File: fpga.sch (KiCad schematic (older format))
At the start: 58 parts, among them P1 JTAG_CONN, SW2 SW_PUSH, U10 S25FL216K, U12 TLV70012, U13 TLV70025, U14 TLV70012, U2 EP4CE15E22

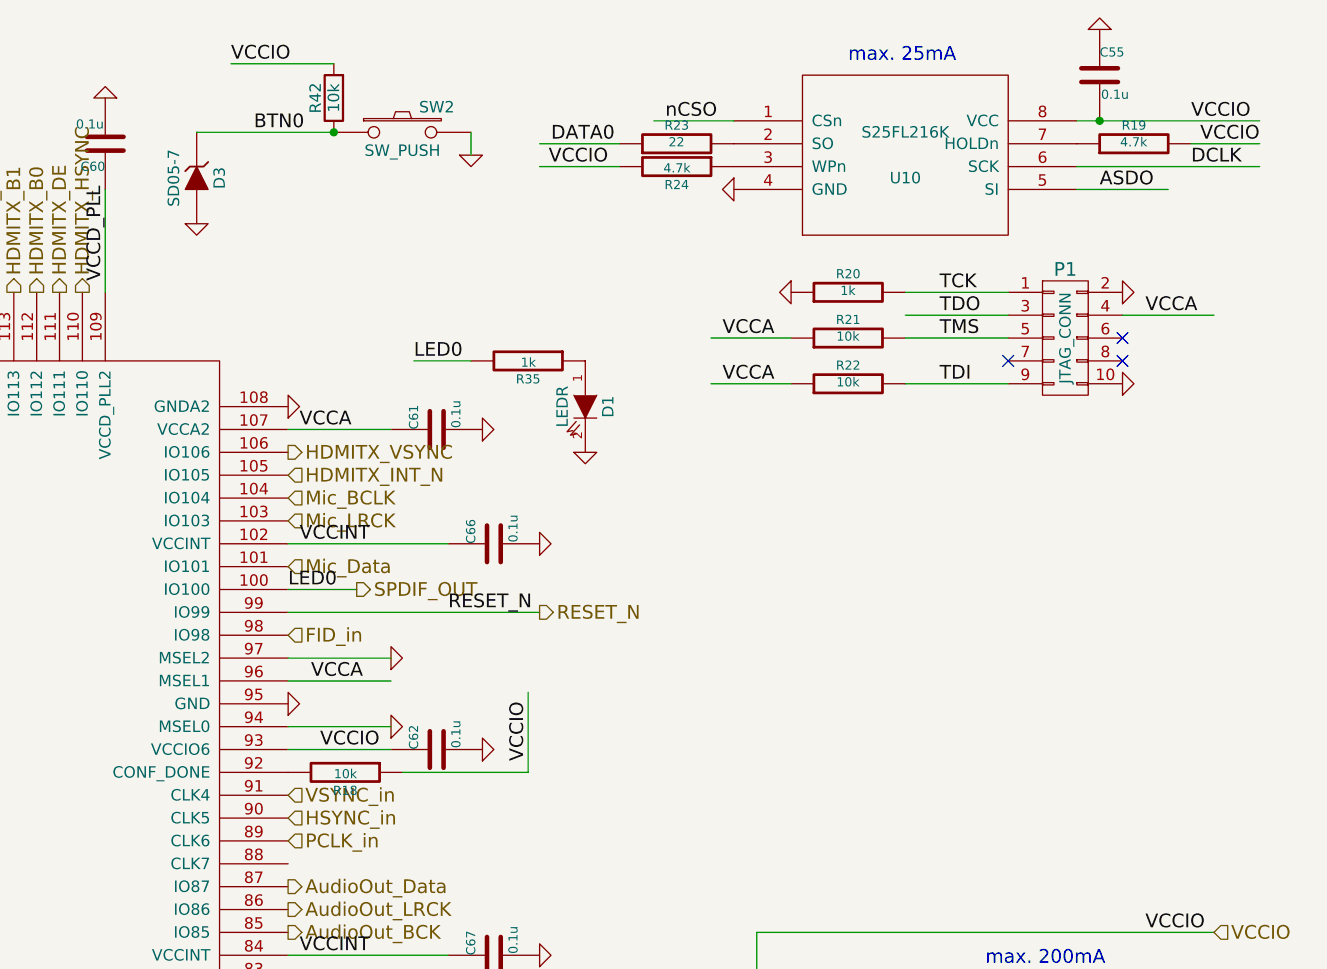
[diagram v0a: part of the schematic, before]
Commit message: update PCB 2
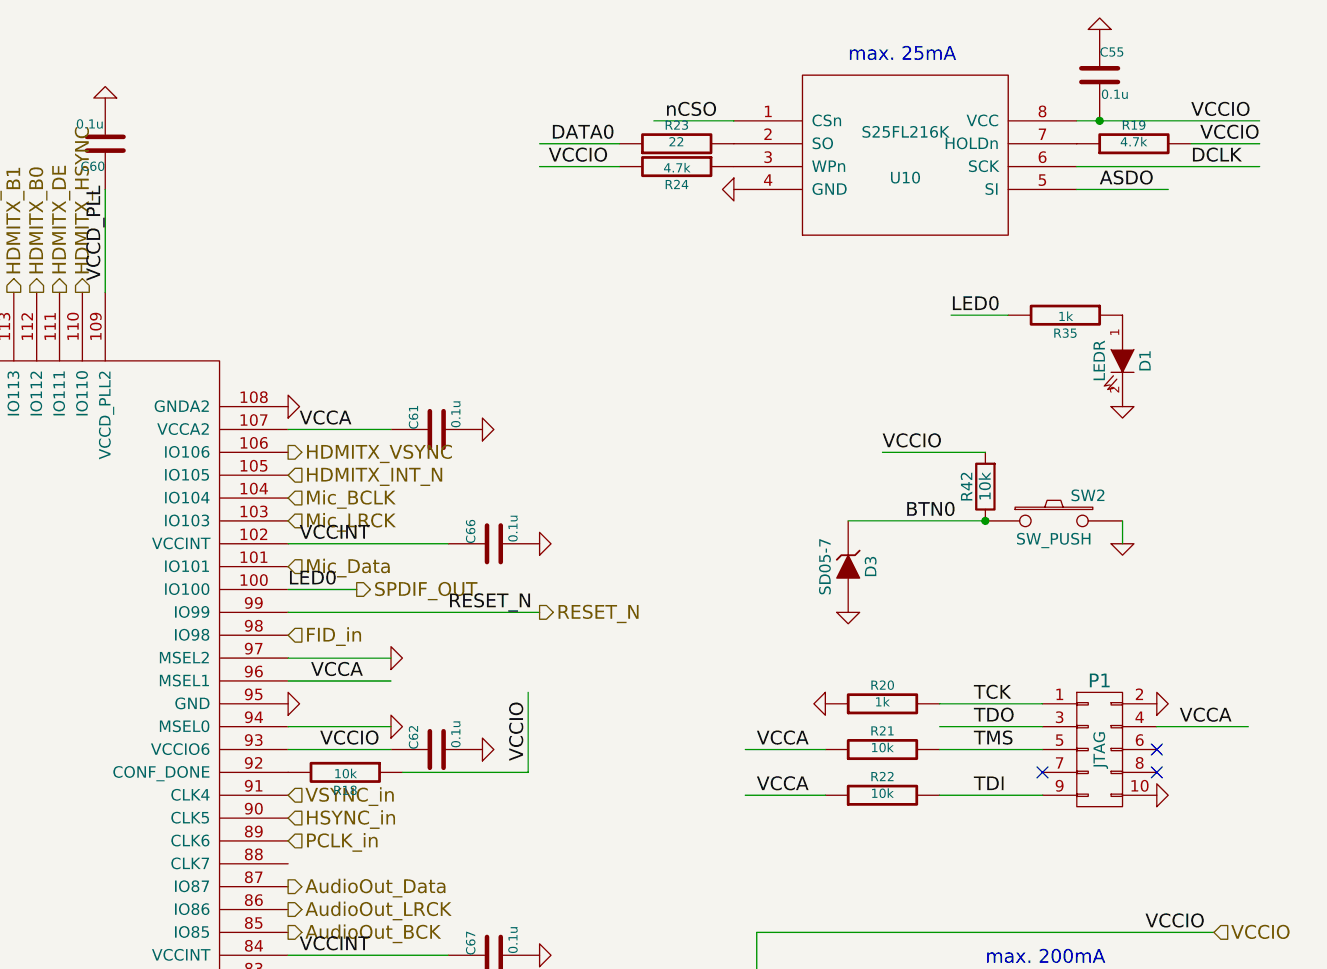
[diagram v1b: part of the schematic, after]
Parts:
- P1: value JTAG_CONN -> JTAG
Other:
- moved on the sheet: D1, D3, P1, R20, R21, R22, R35, R42, SW2
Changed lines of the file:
@@
 L ossc_board-rescue:CONN_02X05 P1
 U 1 1 54FE1877
-P 10200 2050
-F 0 "P1" H 10200 2350 60  0000 C CNN
-F 1 "JTAG_CONN" V 10200 2050 50  0000 C CNN
-F 2 "Connect:VASCH5x2" H 10200 2050 60  0001 C CNN
-F 3 "" H 10200 2050 60  0000 C CNN
-	1    10200 2050
-	1    0    0    -1
-$EndComp
-Text Label 9650 1850 0    60   ~ 0
+P 10350 3850
+F 0 "P1" H 10350 4150 60  0000 C CNN
+F 1 "JTAG" V 10350 3850 50  0000 C CNN
+F 2 "Connect:VASCH5x2" H 10350 3850 60  0001 C CNN
+F 3 "" H 10350 3850 60  0000 C CNN
+	1    10350 3850
+	1    0    0    -1
+$EndComp
+Text Label 9800 3650 0    60   ~ 0
 TCK
-Text Label 9650 1950 0    60   ~ 0
+Text Label 9800 3750 0    60   ~ 0
 TDO
-Text Label 9650 2050 0    60   ~ 0
+Text Label 9800 3850 0    60   ~ 0
 TMS
-Text Label 9650 2250 0    60   ~ 0
+Text Label 9800 4050 0    60   ~ 0
 TDI
 $Comp
 L ossc_board-rescue:GND-RESCUE-ossc_board #PWR048
 U 1 1 54FE19F5
-P 10450 1850
-F 0 "#PWR048" H 10450 1850 30  0001 C CNN
-F 1 "GND" H 10450 1780 30  0001 C CNN
-F 2 "" H 10450 1850 60  0001 C CNN
-F 3 "" H 10450 1850 60  0000 C CNN
-	1    10450 1850
+P 10600 3650
+F 0 "#PWR048" H 10600 3650 30  0001 C CNN
+F 1 "GND" H 10600 3580 30  0001 C CNN
+F 2 "" H 10600 3650 60  0001 C CNN
+F 3 "" H 10600 3650 60  0000 C CNN
+	1    10600 3650
 	0    -1   -1   0
 $EndComp
@@
 L ossc_board-rescue:GND-RESCUE-ossc_board #PWR049
 U 1 1 54FE19FB
-P 10450 2250
-F 0 "#PWR049" H 10450 2250 30  0001 C CNN
-F 1 "GND" H 10450 2180 30  0001 C CNN
-F 2 "" H 10450 2250 60  0001 C CNN
-F 3 "" H 10450 2250 60  0000 C CNN
-	1    10450 2250
+P 10600 4050
+F 0 "#PWR049" H 10600 4050 30  0001 C CNN
+F 1 "GND" H 10600 3980 30  0001 C CNN
+F 2 "" H 10600 4050 60  0001 C CNN
+F 3 "" H 10600 4050 60  0000 C CNN
+	1    10600 4050
 	0    -1   -1   0
 $EndComp
-Text Label 10550 1950 0    60   ~ 0
+Text Label 10700 3750 0    60   ~ 0
 VCCA
 $Comp
 L ossc_board-rescue:R-RESCUE-ossc_board R20
 U 1 1 54FE1A84
-P 9250 1850
-F 0 "R20" V 9330 1850 40  0000 C CNN
-F 1 "1k" V 9257 1851 40  0000 C CNN
-F 2 "Resistor_SMD:R_0603_1608Metric_Pad1.05x0.95mm_HandSolder" V 9180 1850 30  0001 C CNN
-F 3 "~" H 9250 1850 30  0000 C CNN
-	1    9250 1850
+P 9400 3650
+F 0 "R20" V 9480 3650 40  0000 C CNN
+F 1 "1k" V 9407 3651 40  0000 C CNN
+F 2 "Resistor_SMD:R_0603_1608Metric_Pad1.05x0.95mm_HandSolder" V 9330 3650 30  0001 C CNN
+F 3 "~" H 9400 3650 30  0000 C CNN
+	1    9400 3650
 	0    -1   -1   0
 $EndComp
@@
 L ossc_board-rescue:GND-RESCUE-ossc_board #PWR050
 U 1 1 54FE1A96
-P 9000 1850
-F 0 "#PWR050" H 9000 1850 30  0001 C CNN
-F 1 "GND" H 9000 1780 30  0001 C CNN
-F 2 "" H 9000 1850 60  0001 C CNN
-F 3 "" H 9000 1850 60  0000 C CNN
-	1    9000 1850
+P 9150 3650
+F 0 "#PWR050" H 9150 3650 30  0001 C CNN
+F 1 "GND" H 9150 3580 30  0001 C CNN
+F 2 "" H 9150 3650 60  0001 C CNN
+F 3 "" H 9150 3650 60  0000 C CNN
+	1    9150 3650
 	0    1    1    0
 $EndComp
@@
 L ossc_board-rescue:R-RESCUE-ossc_board R21
 U 1 1 54FE1A9C
-P 9250 2050
-F 0 "R21" V 9330 2050 40  0000 C CNN
-F 1 "10k" V 9257 2051 40  0000 C CNN
-F 2 "Resistor_SMD:R_0603_1608Metric_Pad1.05x0.95mm_HandSolder" V 9180 2050 30  0001 C CNN
-F 3 "~" H 9250 2050 30  0000 C CNN
-	1    9250 2050
+P 9400 3850
+F 0 "R21" V 9480 3850 40  0000 C CNN
+F 1 "10k" V 9407 3851 40  0000 C CNN
+F 2 "Resistor_SMD:R_0603_1608Metric_Pad1.05x0.95mm_HandSolder" V 9330 3850 30  0001 C CNN
+F 3 "~" H 9400 3850 30  0000 C CNN
+	1    9400 3850
 	0    -1   -1   0
 $EndComp
@@
 L ossc_board-rescue:R-RESCUE-ossc_board R22
 U 1 1 54FE1AB4
-P 9250 2250
-F 0 "R22" V 9330 2250 40  0000 C CNN
-F 1 "10k" V 9257 2251 40  0000 C CNN
-F 2 "Resistor_SMD:R_0603_1608Metric_Pad1.05x0.95mm_HandSolder" V 9180 2250 30  0001 C CNN
-F 3 "~" H 9250 2250 30  0000 C CNN
-	1    9250 2250
+P 9400 4050
+F 0 "R22" V 9480 4050 40  0000 C CNN
+F 1 "10k" V 9407 4051 40  0000 C CNN
+F 2 "Resistor_SMD:R_0603_1608Metric_Pad1.05x0.95mm_HandSolder" V 9330 4050 30  0001 C CNN
+F 3 "~" H 9400 4050 30  0000 C CNN
+	1    9400 4050
 	0    -1   -1   0
 $EndComp
-Text Label 8700 2050 0    60   ~ 0
+Text Label 8850 3850 0    60   ~ 0
 VCCA
-Text Label 8700 2250 0    60   ~ 0
+Text Label 8850 4050 0    60   ~ 0
 VCCA
 Text Label 1350 3850 0    60   ~ 0
@@
 	1    0    0    -1
 $EndComp
-NoConn ~ 9950 2150
-NoConn ~ 10450 2150
-NoConn ~ 10450 2050
+NoConn ~ 10100 3950
+NoConn ~ 10600 3950
+NoConn ~ 10600 3850
 Text Label 3900 1450 3    60   ~ 0
 VCCIO
@@
 L ossc_board-rescue:LED-RESCUE-ossc_board D1
 U 1 1 550764BB
-P 8100 2350
-F 0 "D1" H 8100 2450 50  0000 C CNN
-F 1 "LEDR" H 8100 2250 50  0000 C CNN
-F 2 "LED_THT:LED_D3.0mm_Horizontal_O1.27mm_Z6.0mm" H 8100 2350 60  0001 C CNN
-F 3 "~" H 8100 2350 60  0000 C CNN
-	1    8100 2350
+P 10450 2150
+F 0 "D1" H 10450 2250 50  0000 C CNN
+F 1 "LEDR" H 10450 2050 50  0000 C CNN
+F 2 "LED_THT:LED_D3.0mm_Horizontal_O1.27mm_Z6.0mm" H 10450 2150 60  0001 C CNN
+F 3 "~" H 10450 2150 60  0000 C CNN
+	1    10450 2150
 	0    1    1    0
 $EndComp
@@
 L ossc_board-rescue:GND-RESCUE-ossc_board #PWR062
 U 1 1 550764C1
-P 8100 2550
-F 0 "#PWR062" H 8100 2550 30  0001 C CNN
-F 1 "GND" H 8100 2480 30  0001 C CNN
-F 2 "" H 8100 2550 60  0001 C CNN
-F 3 "" H 8100 2550 60  0000 C CNN
-	1    8100 2550
+P 10450 2350
+F 0 "#PWR062" H 10450 2350 30  0001 C CNN
+F 1 "GND" H 10450 2280 30  0001 C CNN
+F 2 "" H 10450 2350 60  0001 C CNN
+F 3 "" H 10450 2350 60  0000 C CNN
+	1    10450 2350
 	1    0    0    -1
 $EndComp
@@
 L ossc_board-rescue:R-RESCUE-ossc_board R35
 U 1 1 550764C7
-P 7850 2150
-F 0 "R35" V 7930 2150 40  0000 C CNN
-F 1 "1k" V 7857 2151 40  0000 C CNN
-F 2 "Resistor_SMD:R_0603_1608Metric_Pad1.05x0.95mm_HandSolder" V 7780 2150 30  0001 C CNN
-F 3 "~" H 7850 2150 30  0000 C CNN
-	1    7850 2150
+P 10200 1950
+F 0 "R35" V 10280 1950 40  0000 C CNN
+F 1 "1k" V 10207 1951 40  0000 C CNN
+F 2 "Resistor_SMD:R_0603_1608Metric_Pad1.05x0.95mm_HandSolder" V 10130 1950 30  0001 C CNN
+F 3 "~" H 10200 1950 30  0000 C CNN
+	1    10200 1950
 	0    1    1    0
 $EndComp
-Text Label 7350 2150 0    60   ~ 0
+Text Label 9700 1950 0    60   ~ 0
 LED0
 $Comp
@@
 	900  3150 1200 3150
 Wire Wire Line
-	9500 1850 9950 1850
-Wire Wire Line
-	9500 1950 9950 1950
-Wire Wire Line
-	9500 2050 9950 2050
-Wire Wire Line
-	9500 2250 9950 2250
-Wire Wire Line
-	10450 1950 10850 1950
-Wire Wire Line
-	8650 2050 9000 2050
-Wire Wire Line
-	8650 2250 9000 2250
+	9650 3650 10100 3650
+Wire Wire Line
+	9650 3750 10100 3750
+Wire Wire Line
+	9650 3850 10100 3850
+Wire Wire Line
+	9650 4050 10100 4050
+Wire Wire Line
+	10600 3750 11000 3750
+Wire Wire Line
+	8800 3850 9150 3850
+Wire Wire Line
+	8800 4050 9150 4050
 Wire Wire Line
 	1300 3850 1700 3850
@@
 	1250 5850 1200 5850
 Wire Wire Line
-	7350 2150 7600 2150
+	9700 1950 9950 1950
 Wire Wire Line
 	10050 5450 10050 5400
@@
 L ossc_board-rescue:SW_PUSH SW2
 U 1 1 55EF2D5F
-P 7300 1150
-F 0 "SW2" H 7450 1260 50  0000 C CNN
-F 1 "SW_PUSH" H 7300 1070 50  0000 C CNN
-F 2 "Button_Switch_THT:SW_Tactile_SKHH_Angled" H 7300 1150 60  0001 C CNN
-F 3 "" H 7300 1150 60  0000 C CNN
-	1    7300 1150
+P 10150 2850
+F 0 "SW2" H 10300 2960 50  0000 C CNN
+F 1 "SW_PUSH" H 10150 2770 50  0000 C CNN
+F 2 "Button_Switch_THT:SW_Tactile_SKHH_Angled" H 10150 2850 60  0001 C CNN
+F 3 "" H 10150 2850 60  0000 C CNN
+	1    10150 2850
 	1    0    0    -1
 $EndComp
@@
 L ossc_board-rescue:R R42
 U 1 1 55EF3A70
-P 7000 1000
-F 0 "R42" V 7080 1000 50  0000 C CNN
-F 1 "10k" V 7000 1000 50  0000 C CNN
-F 2 "Resistor_SMD:R_0603_1608Metric_Pad1.05x0.95mm_HandSolder" V 6930 1000 30  0001 C CNN
-F 3 "" H 7000 1000 30  0000 C CNN
-	1    7000 1000
+P 9850 2700
+F 0 "R42" V 9930 2700 50  0000 C CNN
+F 1 "10k" V 9850 2700 50  0000 C CNN
+F 2 "Resistor_SMD:R_0603_1608Metric_Pad1.05x0.95mm_HandSolder" V 9780 2700 30  0001 C CNN
+F 3 "" H 9850 2700 30  0000 C CNN
+	1    9850 2700
 	-1   0    0    1
 $EndComp
 Wire Wire Line
-	6400 1150 7000 1150
-Text Label 6650 1150 0    60   ~ 0
+	9250 2850 9850 2850
+Text Label 9500 2850 0    60   ~ 0
 BTN0
 Wire Wire Line
-	7000 850  6550 850
-Text Label 6550 850  0    60   ~ 0
+	9850 2550 9400 2550
+Text Label 9400 2550 0    60   ~ 0
 VCCIO
 Text Label 1300 4550 2    60   ~ 0
@@
 L ossc_board-rescue:ZENER D3
 U 1 1 58C560B1
-P 6400 1350
-F 0 "D3" H 6400 1450 50  0000 C CNN
-F 1 "SD05-7" H 6400 1250 50  0000 C CNN
-F 2 "custom_components:SOD-323_Handsoldering" H 6400 1350 60  0001 C CNN
-F 3 "" H 6400 1350 60  0000 C CNN
-	1    6400 1350
+P 9250 3050
+F 0 "D3" H 9250 3150 50  0000 C CNN
+F 1 "SD05-7" H 9250 2950 50  0000 C CNN
+F 2 "custom_components:SOD-323_Handsoldering" H 9250 3050 60  0001 C CNN
+F 3 "" H 9250 3050 60  0000 C CNN
+	1    9250 3050
 	0    1    1    0
 $EndComp
@@
 L ossc_board-rescue:GND-RESCUE-ossc_board #PWR078
 U 1 1 58C561E6
-P 6400 1550
-F 0 "#PWR078" H 6400 1550 30  0001 C CNN
-F 1 "GND" H 6400 1480 30  0001 C CNN
-F 2 "" H 6400 1550 60  0001 C CNN
-F 3 "" H 6400 1550 60  0000 C CNN
-	1    6400 1550
+P 9250 3250
+F 0 "#PWR078" H 9250 3250 30  0001 C CNN
+F 1 "GND" H 9250 3180 30  0001 C CNN
+F 2 "" H 9250 3250 60  0001 C CNN
+F 3 "" H 9250 3250 60  0000 C CNN
+	1    9250 3250
 	1    0    0    -1
 $EndComp
@@
 L ossc_board-rescue:GND-RESCUE-ossc_board #PWR0209
 U 1 1 5F7F3064
-P 7600 1250
-F 0 "#PWR0209" H 7600 1250 30  0001 C CNN
-F 1 "GND" H 7600 1180 30  0001 C CNN
-F 2 "" H 7600 1250 60  0001 C CNN
-F 3 "" H 7600 1250 60  0000 C CNN
-	1    7600 1250
-	1    0    0    -1
-$EndComp
-Wire Wire Line
-	7600 1150 7600 1250
-Connection ~ 7000 1150
+P 10450 2950
+F 0 "#PWR0209" H 10450 2950 30  0001 C CNN
+F 1 "GND" H 10450 2880 30  0001 C CNN
+F 2 "" H 10450 2950 60  0001 C CNN
+F 3 "" H 10450 2950 60  0000 C CNN
+	1    10450 2950
+	1    0    0    -1
+$EndComp
+Wire Wire Line
+	10450 2850 10450 2950
+Connection ~ 9850 2850
 Wire Wire Line
 	5000 6350 5000 6800

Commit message: update3
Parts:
- D3: footprint custom_components:SOD-323_Handsoldering -> Diode_SMD:D_SOD-323_HandSoldering
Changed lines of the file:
@@
 F 0 "D3" H 9250 3150 50  0000 C CNN
 F 1 "SD05-7" H 9250 2950 50  0000 C CNN
-F 2 "custom_components:SOD-323_Handsoldering" H 9250 3050 60  0001 C CNN
+F 2 "Diode_SMD:D_SOD-323_HandSoldering" H 9250 3050 60  0001 C CNN
 F 3 "" H 9250 3050 60  0000 C CNN
 	1    9250 3050
